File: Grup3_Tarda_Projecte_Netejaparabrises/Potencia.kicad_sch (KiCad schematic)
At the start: 43 parts, among them J6 CONNECTOR ALIMENTACIO, K1 1393280-6, K2 1393280-6, K3 1393280-6, K4 1393280-6, K5 1393280-6, K6 1393280-6, K8 1393280-6, Q1 BC817-25_RF, Q2 BC817-25_RF, Q3 BC817-25_RF, Q4 BC817-25_RF, Q5 BC817-25_RF, Q6 BC817-25_RF, Q7 BC817-25_RF

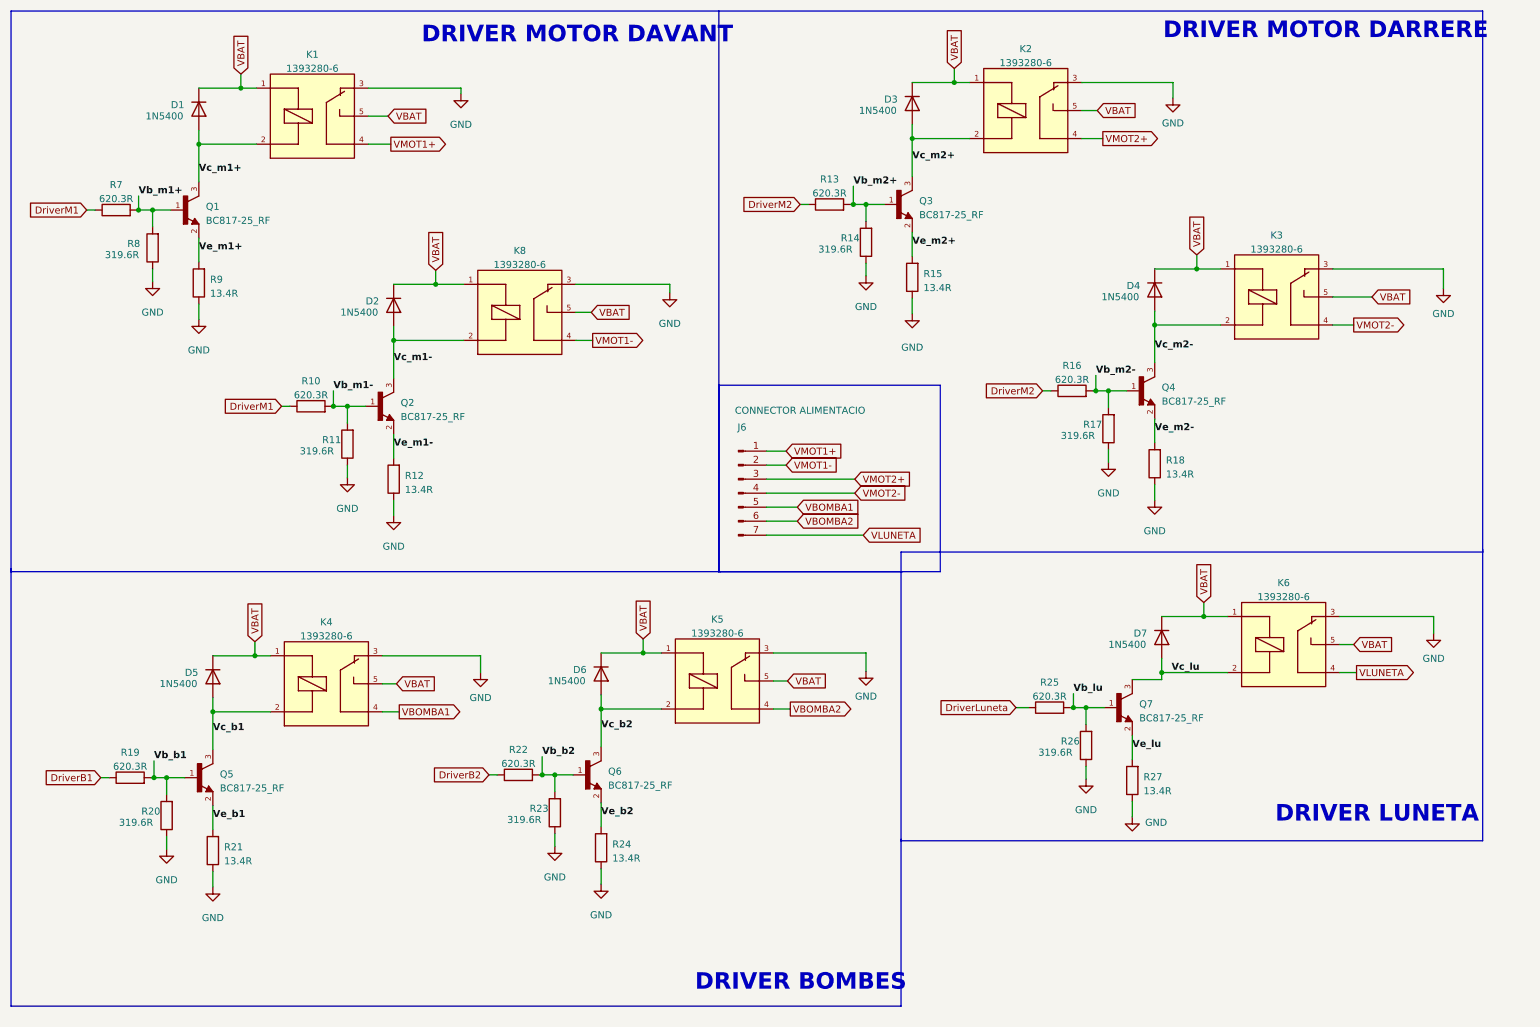
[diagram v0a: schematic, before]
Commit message: canvis reles 07-04-2023
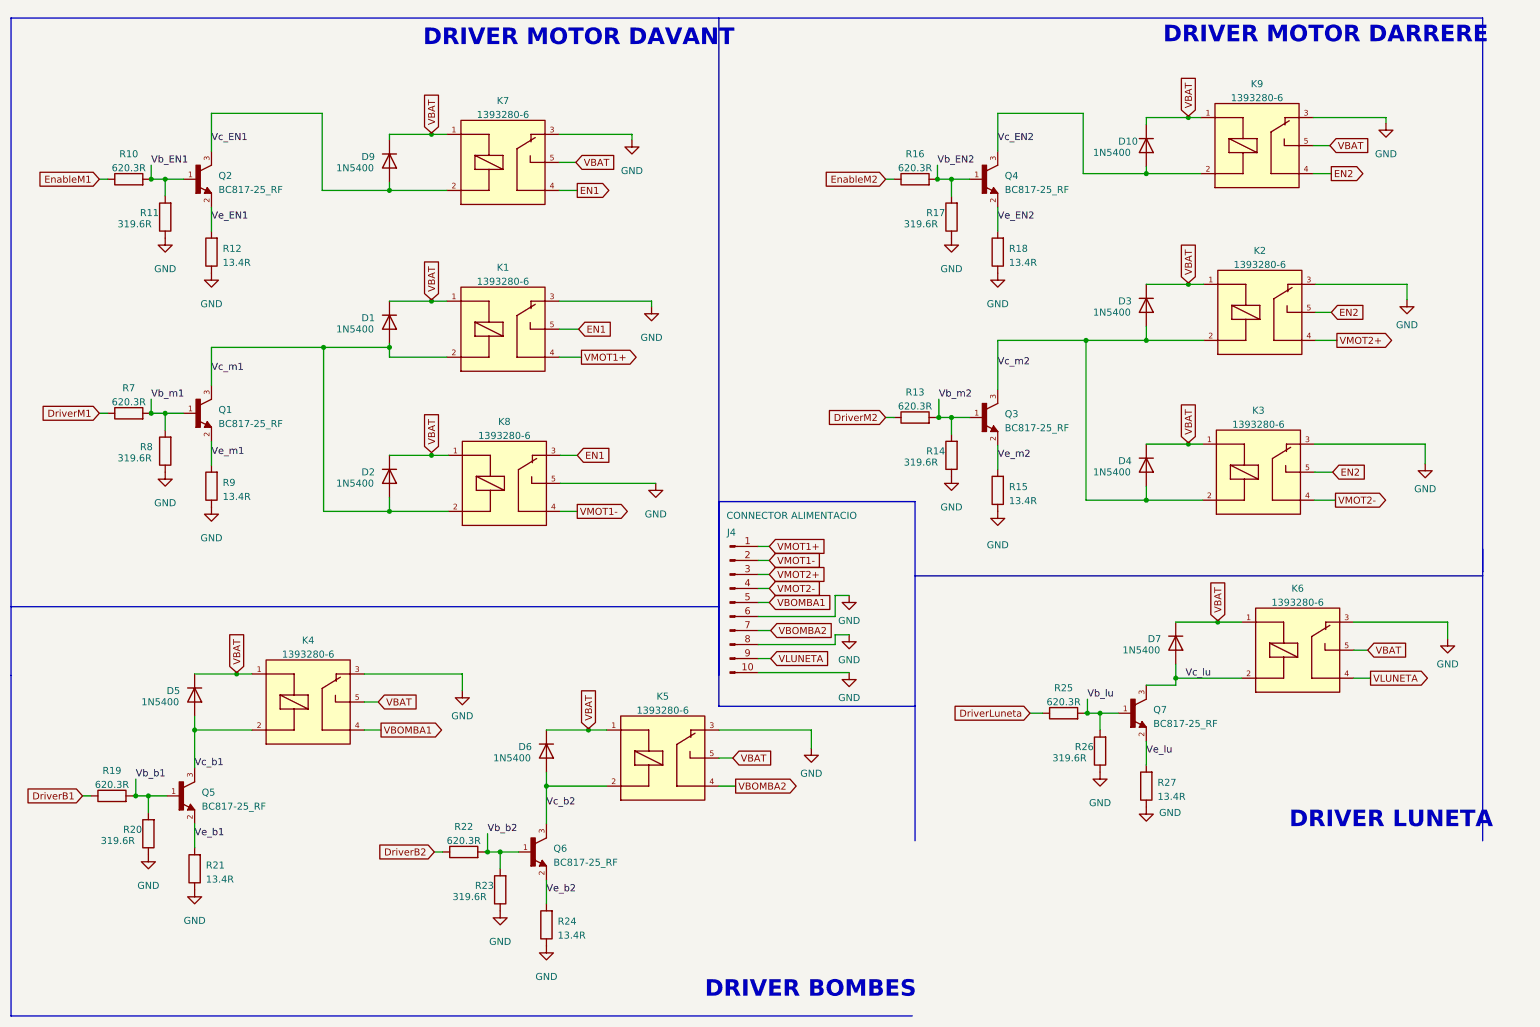
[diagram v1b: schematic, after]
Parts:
- removed J6: CONNECTOR ALIMENTACIO, symbol Connector:Conn_01x07_Pin
- added D10, D9: 1N5400, Diode_THT:D_DO-201AD_P15.24mm_Horizontal, symbol Diode:1N5400
- added J4: CONNECTOR ALIMENTACIO, symbol Connector:Conn_01x10_Pin
- added K7, K9: 1393280-6, RELAY_1393280-6, symbol 1393280-6:1393280-6
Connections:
- net DriverM1: no longer R10.1
- net DriverM2: no longer R16.1
- net GND: now also K8.5, J4.10 (Pin_10), J4.6 (Pin_6), J4.8 (Pin_8), K7.3, K9.3; no longer K8.3
- net VBAT: now also D10.1 (K), D9.1 (K), K7.1, K7.5, K9.1, K9.5; no longer K1.5, K2.5, K3.5, K8.5
- net VBOMBA1: now also J4.5 (Pin_5)
- net VBOMBA2: now also J4.7 (Pin_7)
- net VLUNETA: now also J4.9 (Pin_9)
- net VMOT1+: now also J4.1 (Pin_1)
- net VMOT1-: now also J4.2 (Pin_2)
- net VMOT2+: now also J4.3 (Pin_3)
- net VMOT2-: now also J4.4 (Pin_4)
- net Vb_m1+ renamed Vb_m1
- net Vb_m1- renamed Vb_EN1
- net Vb_m2+ renamed Vb_m2
- net Vb_m2- renamed Vb_EN2
- net Vc_m1+ renamed Vc_m1
- net Vc_m1: now also D2.2 (A), K8.2
- removed net Vc_m1-: D2.2 (A), K8.2, Q2.3
- net Vc_m2+ renamed Vc_m2
- net Vc_m2: now also D4.2 (A), K3.2
- removed net Vc_m2-: D4.2 (A), K3.2, Q4.3
- net Ve_m1+ renamed Ve_m1
- net Ve_m1- renamed Ve_EN1
- net Ve_m2+ renamed Ve_m2
- net Ve_m2- renamed Ve_EN2
- new net EN1: K1.5, K7.4, K8.3
- new net EN2: K2.5, K3.5, K9.4
- new net EnableM1: R10.1
- new net EnableM2: R16.1
- new net Vc_EN1: D9.2 (A), K7.2, Q2.3
- new net Vc_EN2: D10.2 (A), K9.2, Q4.3
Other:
- moved on the sheet: D1, D2, D3, D4, D5, D6, D7, K1, K2, K3, K4, K5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
